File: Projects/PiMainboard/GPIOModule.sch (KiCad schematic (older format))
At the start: 0 parts

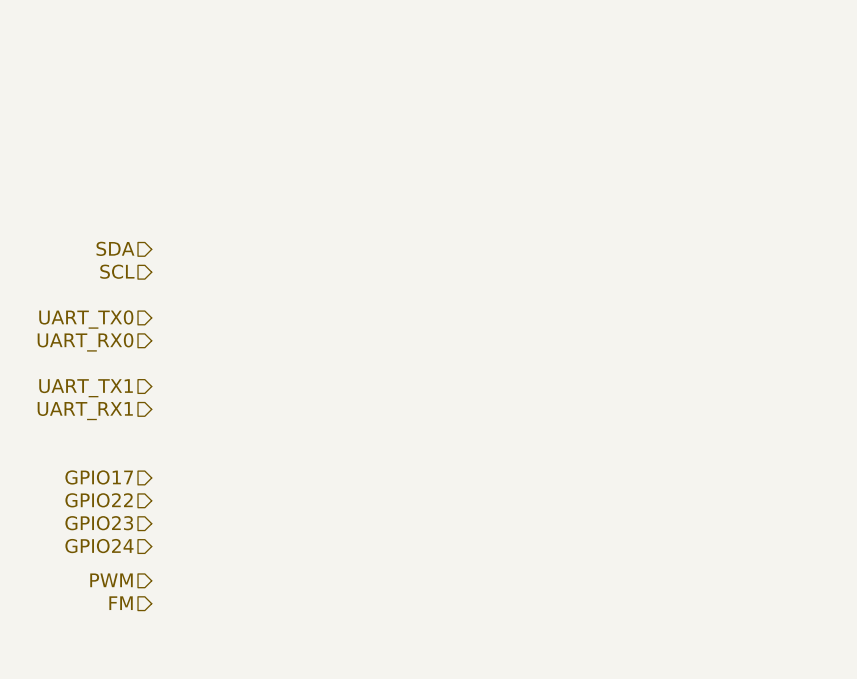
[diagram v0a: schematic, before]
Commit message: Added lots more to modules!
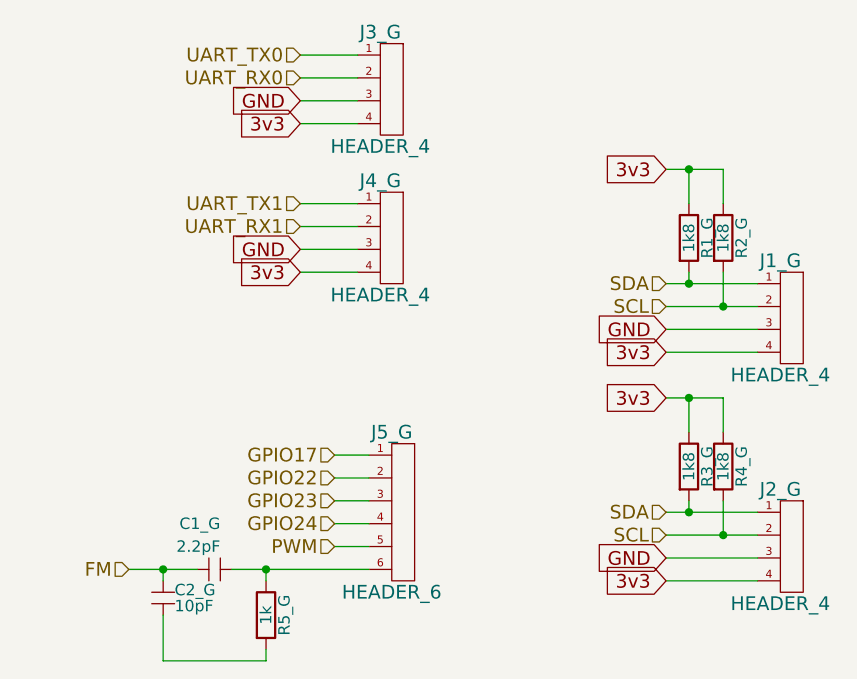
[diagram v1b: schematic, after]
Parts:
- added C1_G: 2.2pF, symbol cap_np
- added C2_G: 10pF, symbol cap_np
- added J1_G, J2_G, J3_G, J4_G: HEADER_4, symbol HEADER_4
- added J5_G: HEADER_6, symbol HEADER_6
- added R1_G, R2_G, R3_G, R4_G: 1k8, symbol R
- added R5_G: 1k, symbol R
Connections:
- net FM: now also C1_G.1, C2_G.1
- net GPIO17: now also J5_G.1
- net GPIO22: now also J5_G.2
- net GPIO23: now also J5_G.3
- net GPIO24: now also J5_G.4
- net PWM: now also J5_G.5
- net SCL: now also J1_G.2, J2_G.2, R2_G.2, R4_G.2
- net SDA: now also J1_G.1, J2_G.1, R1_G.2, R3_G.2
- net UART_RX0: now also J3_G.2
- net UART_RX1: now also J4_G.2
- net UART_TX0: now also J3_G.1
- net UART_TX1: now also J4_G.1
- new net: C1_G.2, J5_G.6, R5_G.1
- new net: C2_G.2, R5_G.2
- new net 3v3: J1_G.4, J2_G.4, J3_G.4, J4_G.4, R1_G.1, R2_G.1, R3_G.1, R4_G.1
- new net GND: J1_G.3, J2_G.3, J3_G.3, J4_G.3
